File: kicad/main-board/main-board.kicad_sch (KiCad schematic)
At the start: 2 parts, among them J1 Conn_01x02, U1 CM5108064B

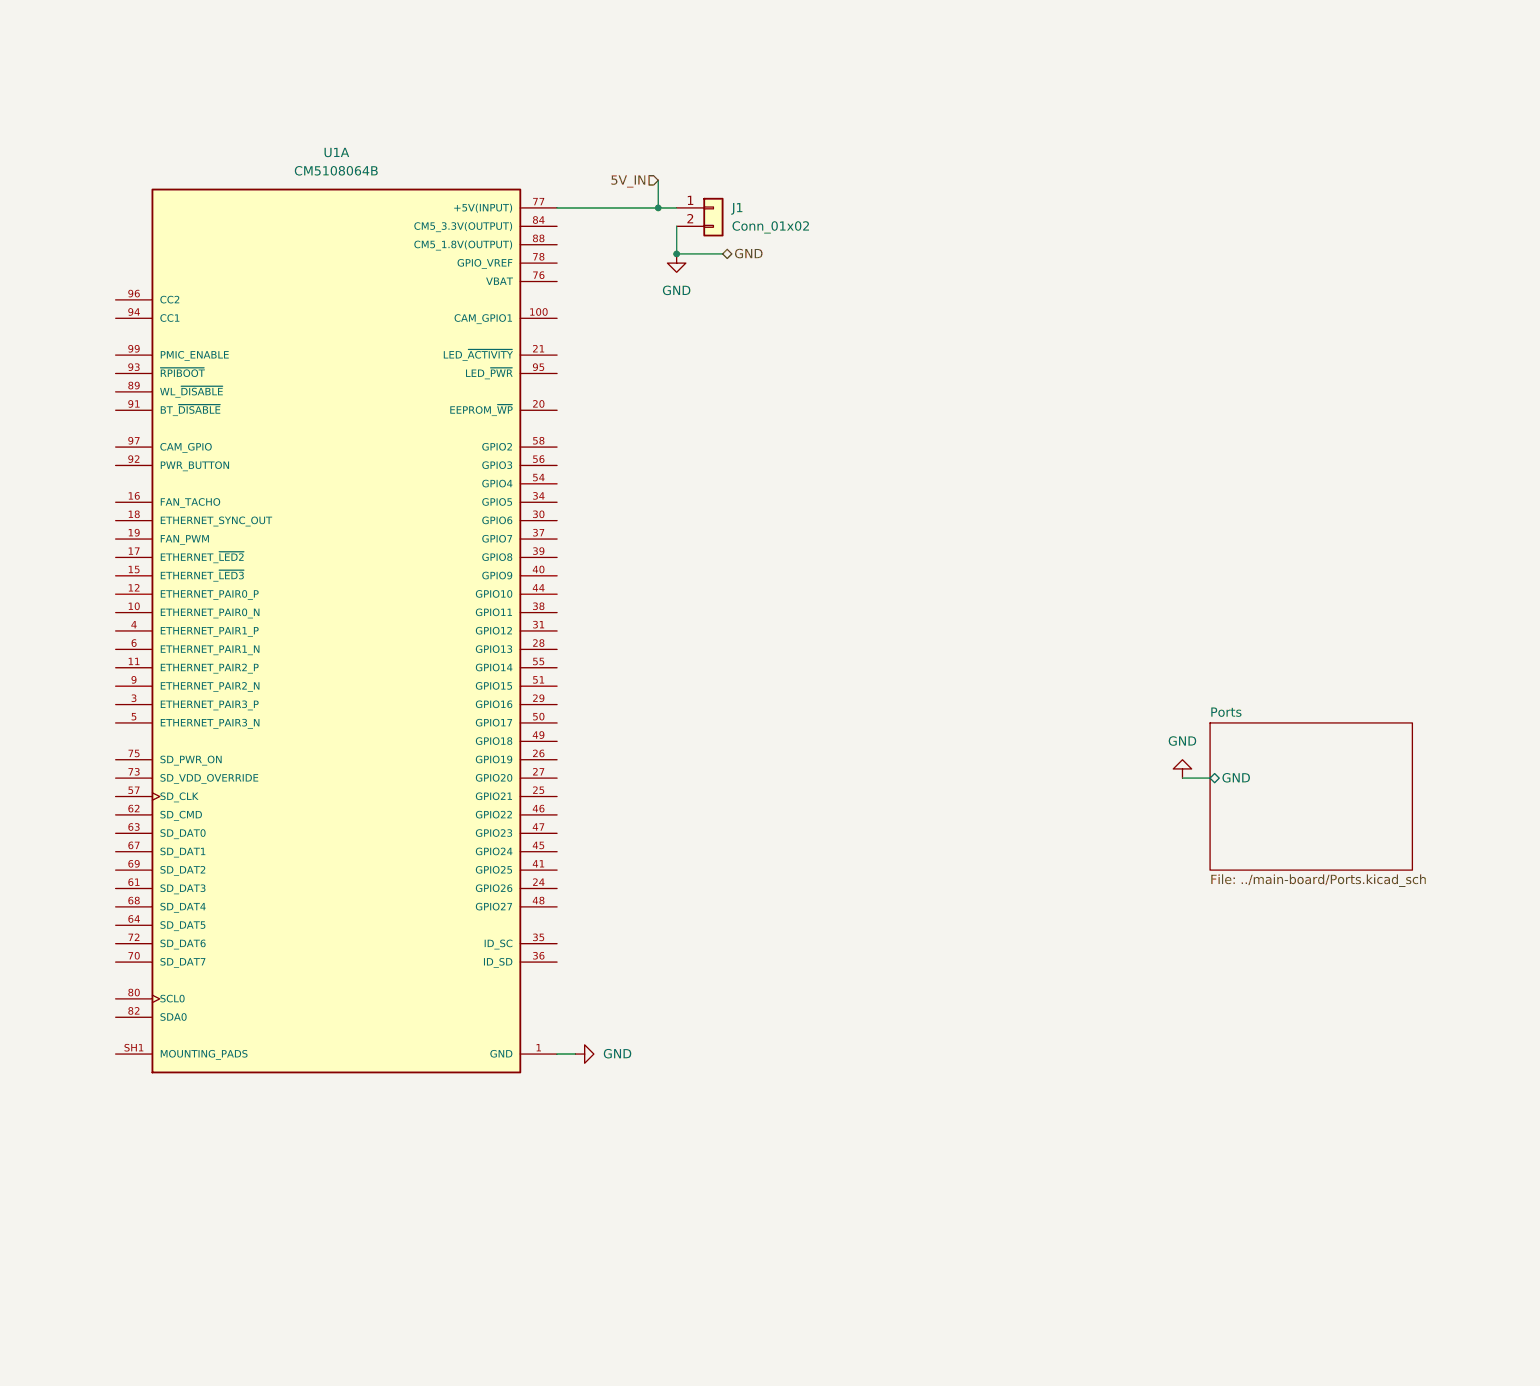
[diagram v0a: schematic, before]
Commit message: worked on main board
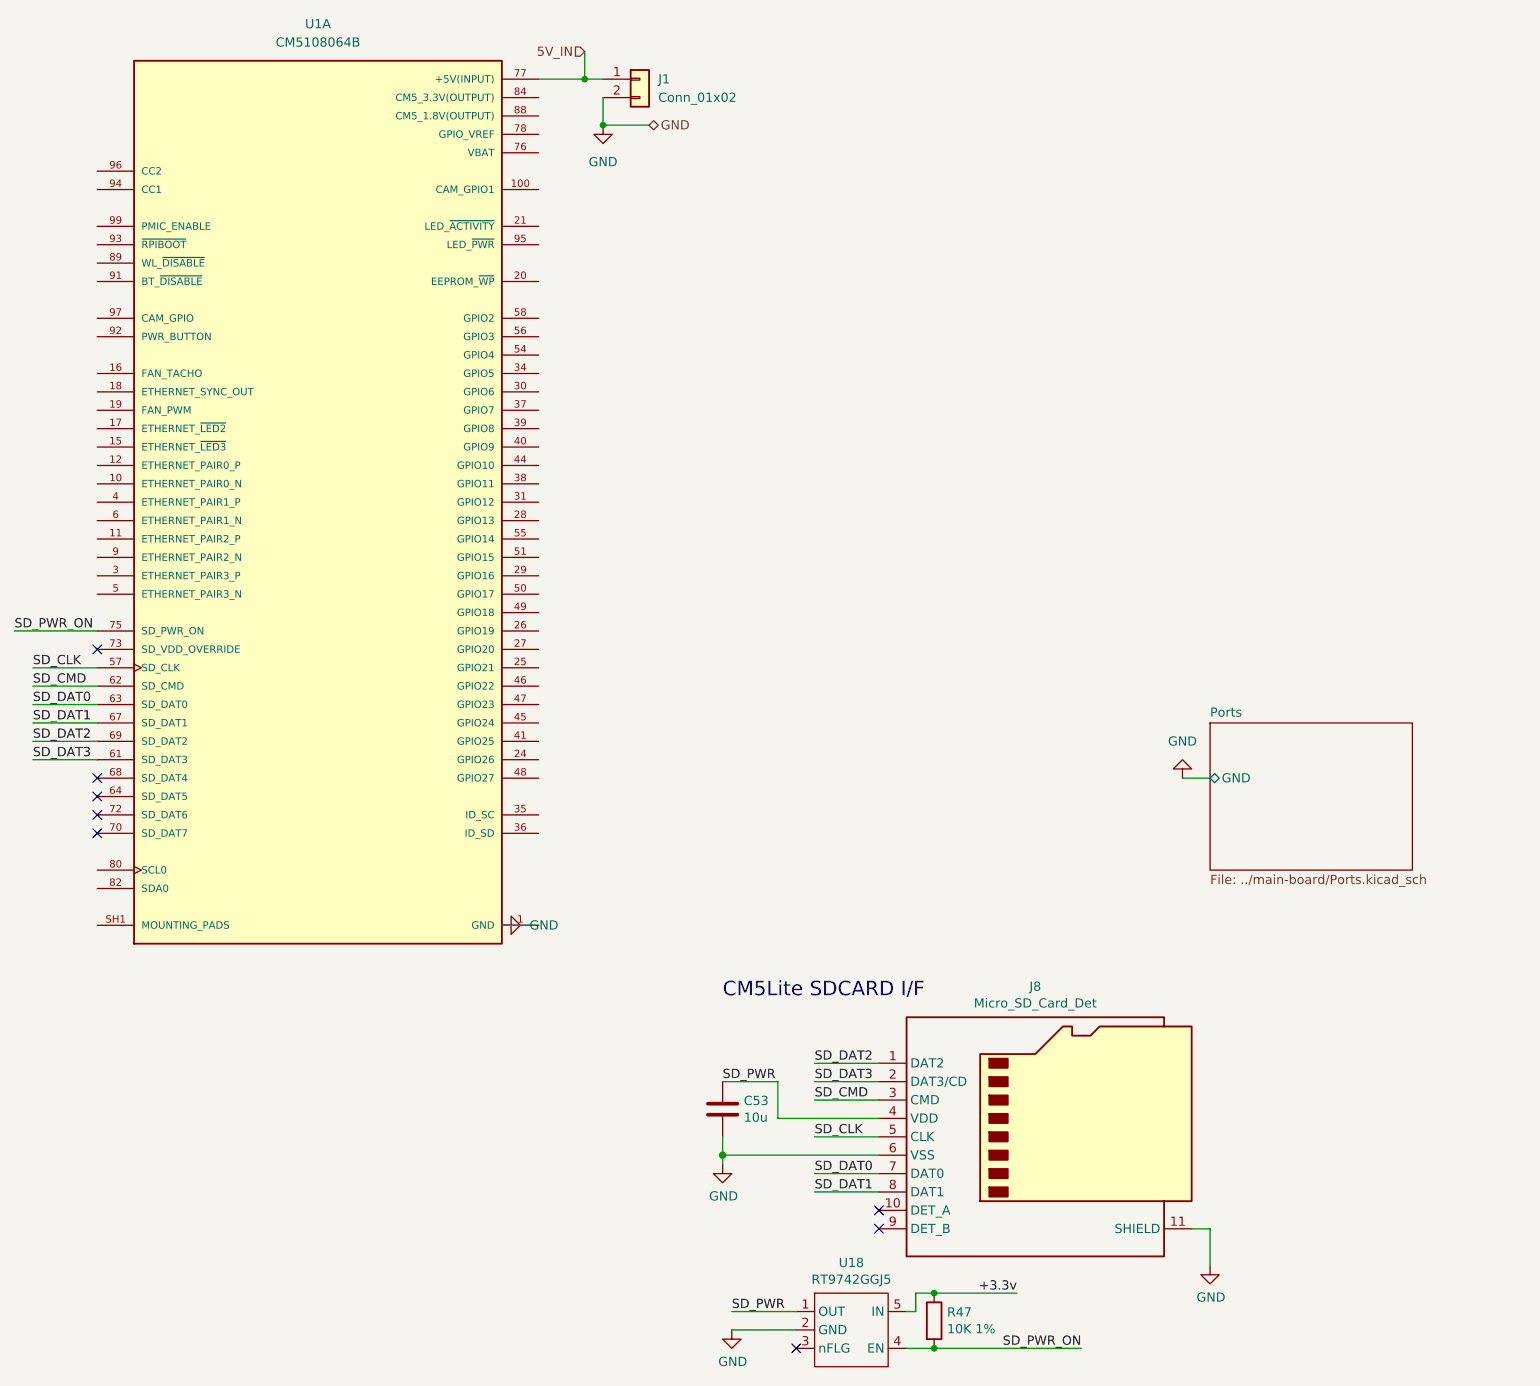
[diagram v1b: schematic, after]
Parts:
- added C53: 10u, Capacitor_SMD:C_0805_2012Metric, symbol Device:C
- added J8: Micro_SD_Card_Det, CM5IO:SDCARD_MOLEX_503398-1892, symbol Connector:Micro_SD_Card_Det2
- added R47: 10K 1%, Resistor_SMD:R_0402_1005Metric, symbol Device:R
- added U18: RT9742GGJ5, Package_TO_SOT_SMD:SOT-23-5, symbol CM5IO:RT9742GGJ5
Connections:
- net GND: now also C53.2, J8.11 (SHIELD), J8.6 (VSS), U18.2 (GND)
- net SD_CLK: now reaches U1.57 (SD_CLK)
- net SD_CLK: now also J8.5 (CLK)
- net SD_DAT3: now reaches U1.61 (SD_DAT3)
- net SD_DAT3: now also J8.2 (DAT3/CD)
- net SD_CMD: now reaches U1.62 (SD_CMD)
- net SD_CMD: now also J8.3 (CMD)
- net SD_DAT0: now reaches U1.63 (SD_DAT0)
- net SD_DAT0: now also J8.7 (DAT0)
- net SD_DAT1: now reaches U1.67 (SD_DAT1)
- net SD_DAT1: now also J8.8 (DAT1)
- net SD_DAT2: now reaches U1.69 (SD_DAT2)
- net SD_DAT2: now also J8.1 (DAT2)
- net SD_PWR_ON: now reaches U1.75 (SD_PWR_ON)
- net SD_PWR_ON: now also R47.2, U18.4 (EN)
- new net +3.3v: R47.1, U18.5 (IN)
- new net SD_PWR: C53.1, J8.4 (VDD), U18.1 (OUT)
- no-connect marks 0 -> 8
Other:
- note added: "CM5Lite SDCARD I/F"
- moved on the sheet: J1, U1A
